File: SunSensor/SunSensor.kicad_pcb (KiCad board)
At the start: 2 copper layers, 16 parts, among them U1 AD7291BCPZ

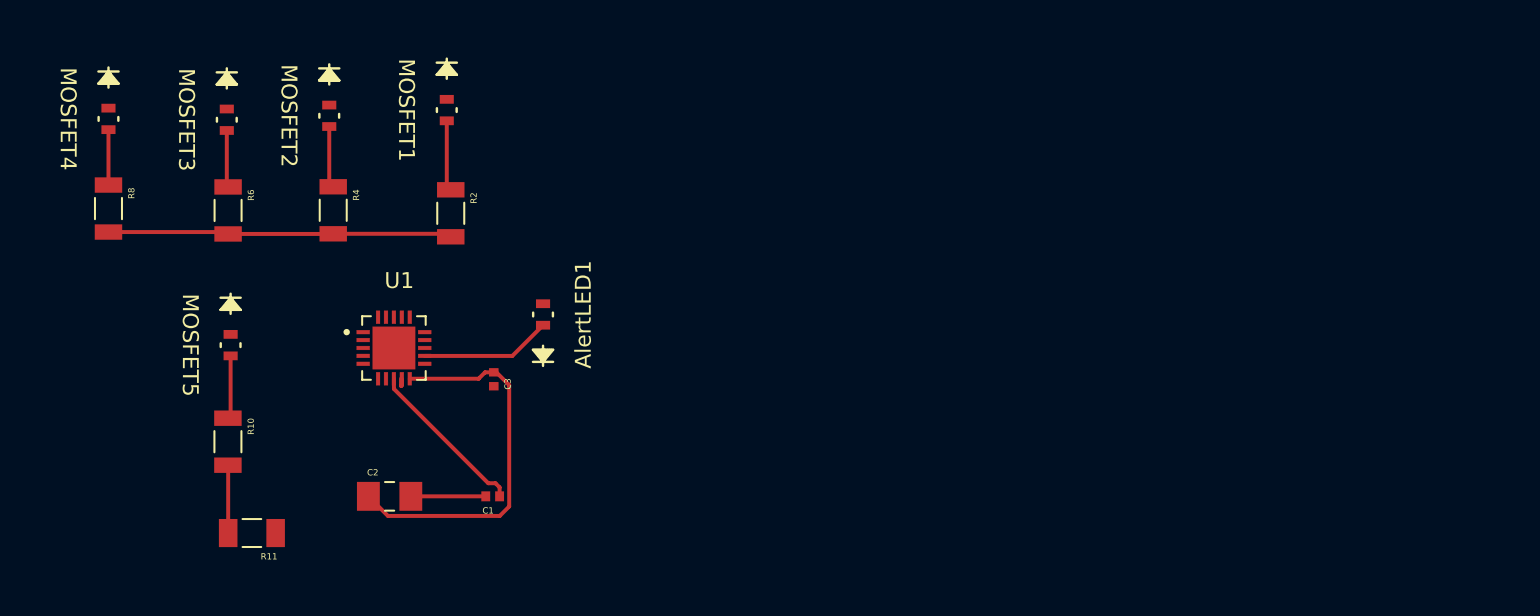
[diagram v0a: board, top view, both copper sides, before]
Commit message: Finished traces
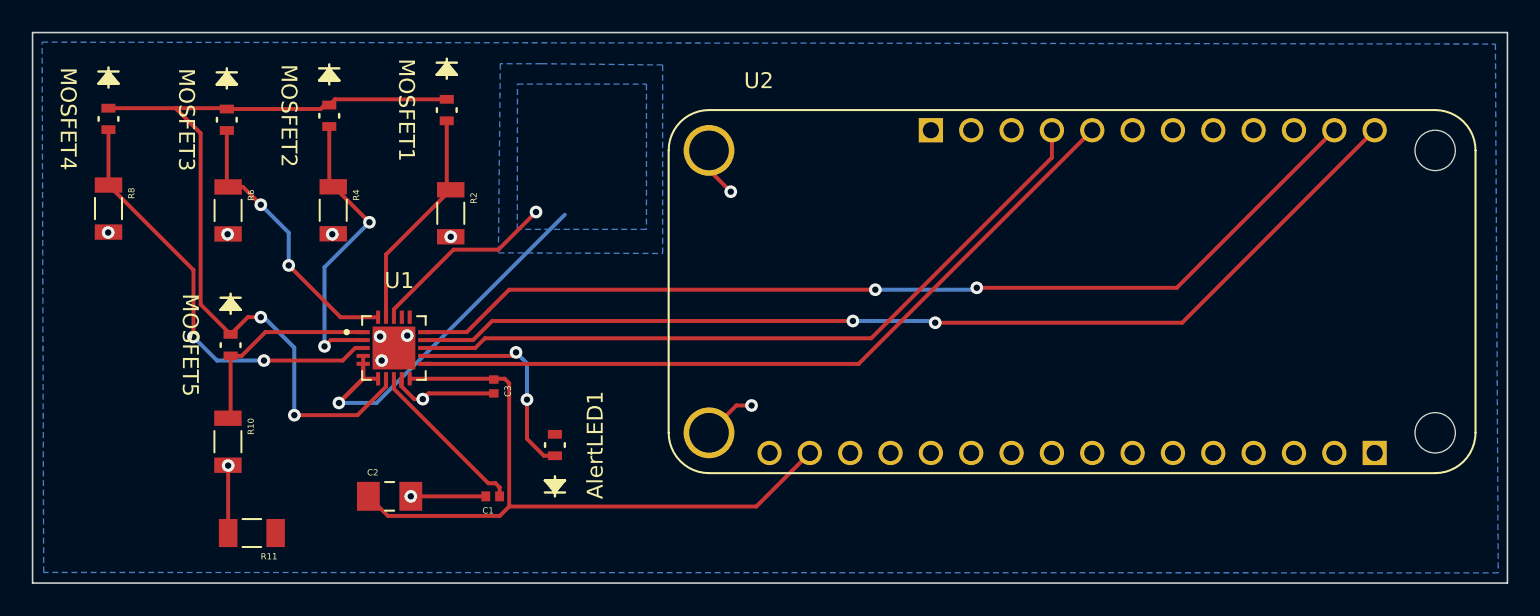
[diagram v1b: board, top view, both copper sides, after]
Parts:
- added U2: FEATHER_M0_BASIC_PROTO, sunsensor:MODULE_FEATHER_M0_BASIC_PROTO, F.Cu at (165.4, 98.4)
- moved AlertLED1 8.25 mm to (132.8, 108.1)
- moved C3 0.45 mm to (129.0, 104.4)
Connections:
- C1 pad 2: GNDS -> GNDREF
- C2 pad 2: GNDS -> GNDREF
- C3 pad 2: GNDS -> GNDREF
- U1 pad 11: unconnected-(U1-Pad11) -> /AS0
- U1 pad 13: unconnected-(U1-Pad13) -> /AS1
- U1 pad 14: unconnected-(U1-Pad14) -> /SDA_chip
- U1 pad 15: unconnected-(U1-Pad15) -> /SCL_chip
- U1 pad 16: unconnected-(U1-Pad16) -> +3V3
- U1 pad 21: (no net) -> GNDREF
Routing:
- net /SDA_chip: track 0.00 -> 65.4 mm, vias 0 -> 2
- net /SCL_chip: track 0.00 -> 62.5 mm, vias 0 -> 2
- net /V_ref: track 0.00 -> 53.8 mm, vias 0 -> 2
- net /AS0: track 0.00 -> 48.1 mm
- net /AS1: track 0.00 -> 46.2 mm
- net GNDS: track 4.72 -> 38.7 mm, vias 0 -> 2
- net /Vin5: track 3.49 -> 26.9 mm, vias 0 -> 2
- net +3V3: track 24.0 -> 44.1 mm
- net /Vin4: track 3.90 -> 18.7 mm, vias 0 -> 2
- net /Vin2: track 3.59 -> 17.6 mm, vias 0 -> 2
- net /Vin1: track 4.45 -> 14.2 mm
- net /Vin3: track 3.99 -> 13.0 mm
- net Net-(AlertLED1-Pad1): track 8.25 -> 13.8 mm, vias 0 -> 2
- net GNDREF: track 26.9 -> 22.8 mm, vias 0 -> 12
- added copper zone on B.Cu, net GNDREF
- added copper zone on B.Cu, net GNDS
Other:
- board outline added: 92.9 x 34.7 mm
